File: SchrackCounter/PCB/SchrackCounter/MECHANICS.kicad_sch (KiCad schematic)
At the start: 24 parts, among them J3 Conn_01x02_Pin, J4 Conn_01x02_Pin, J5 MEM2067-02-180-00-A_REVB, M1 Fan_CPU_4pin, SW1 SW_Push, SW2 SW_Push, SW3 SW_Push, SW4 SW_Push

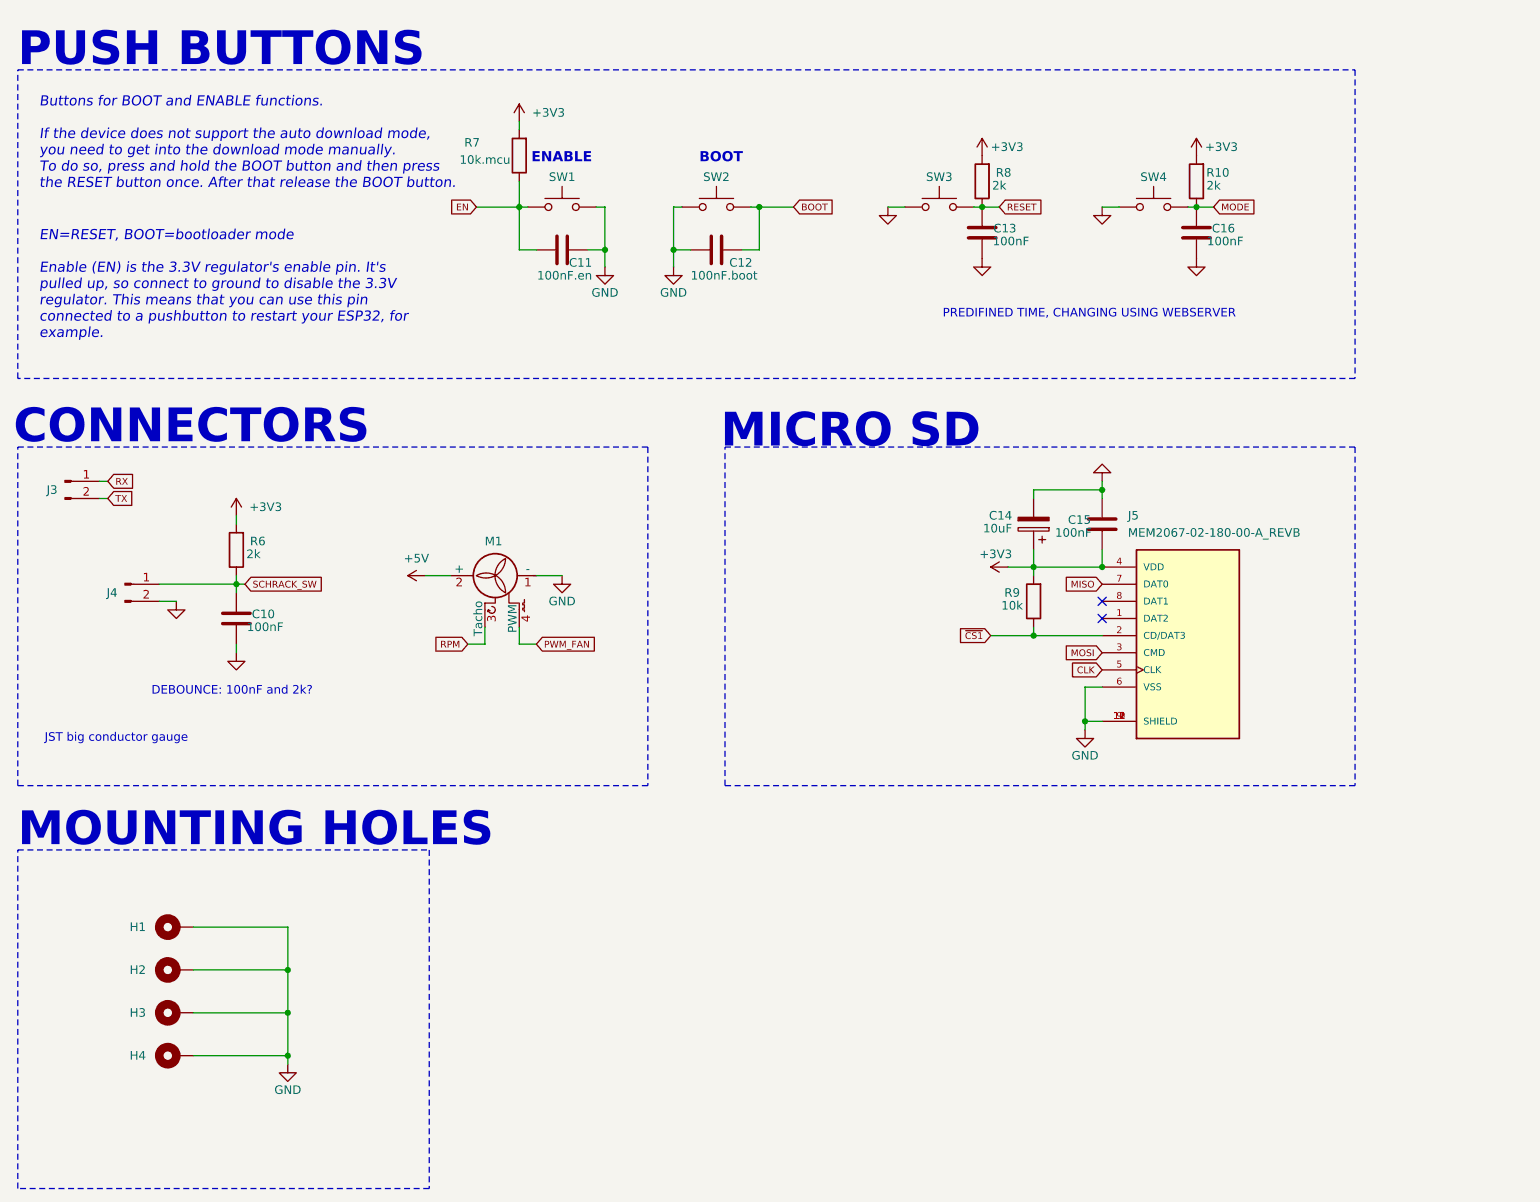
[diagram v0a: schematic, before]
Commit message: PCB layout update
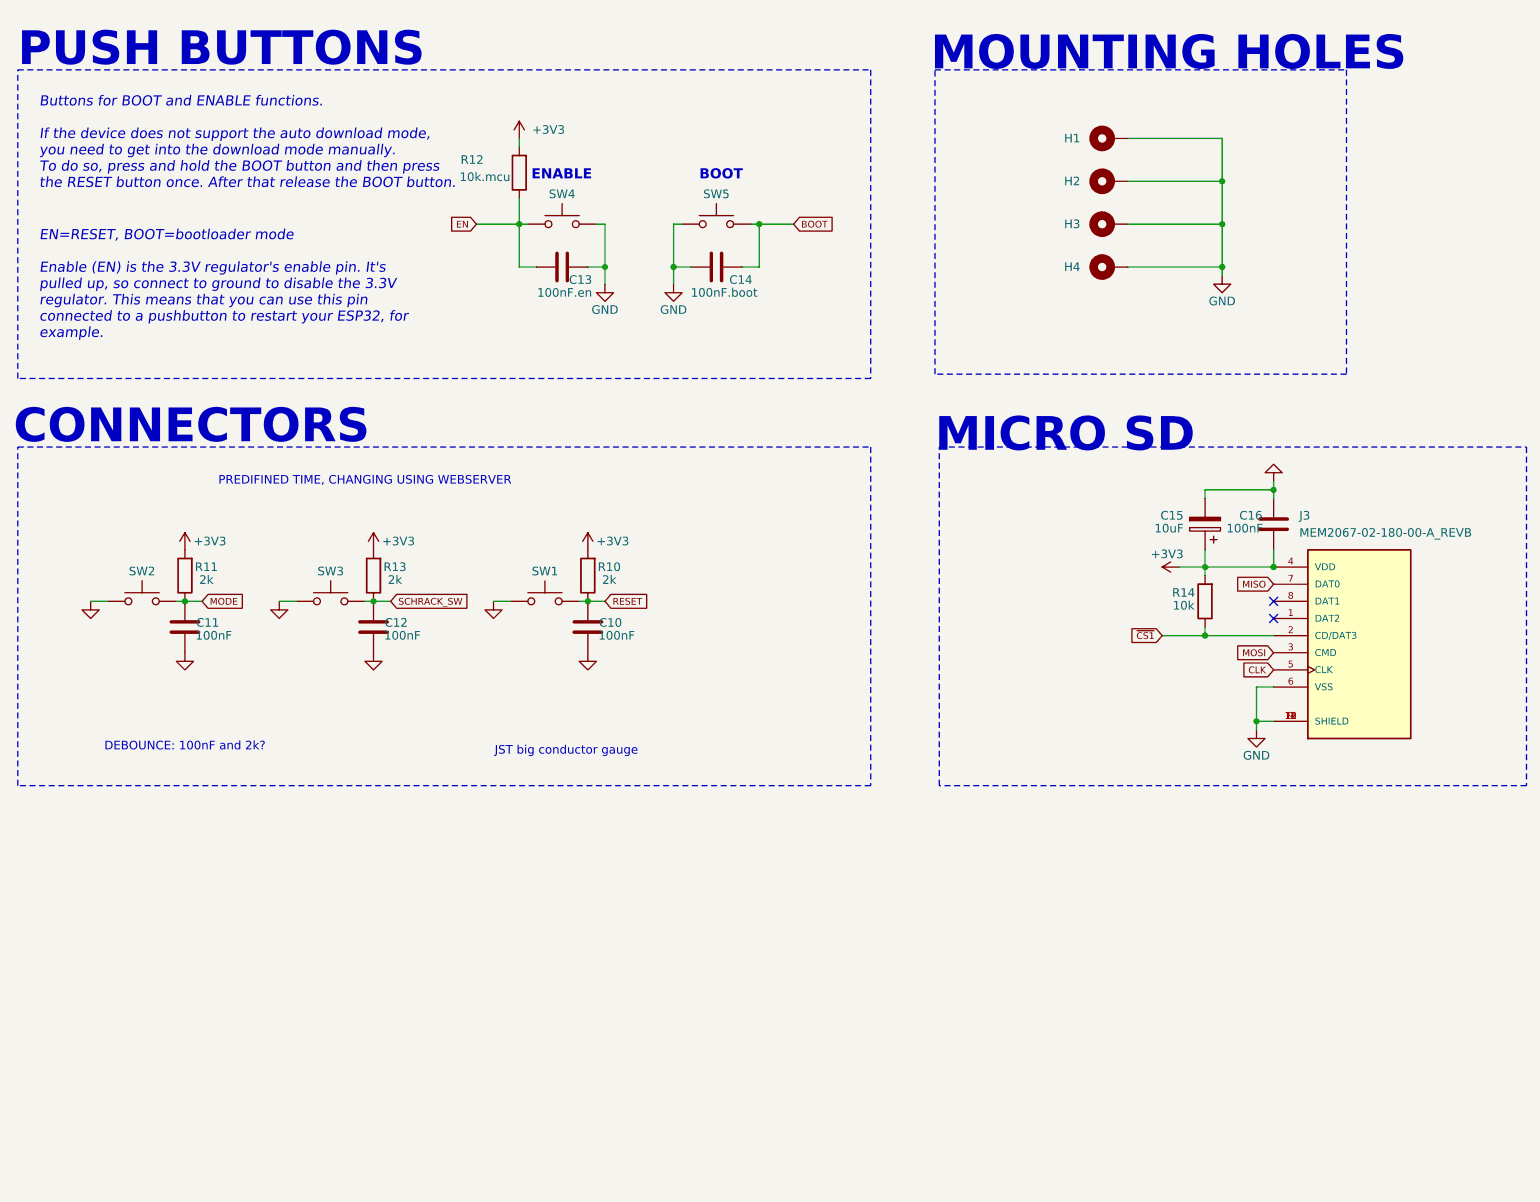
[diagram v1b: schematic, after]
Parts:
- removed J3: Conn_01x02_Pin, Connector_PinHeader_2.54mm:PinHeader_1x02_P2.54mm_Vertical, symbol Connector:Conn_01x02_Pin
- removed J4: Conn_01x02_Pin, Connector_JST:JST_XH_B2B-XH-A_1x02_P2.50mm_Vertical, symbol Connector:Conn_01x02_Pin
- removed M1: Fan_CPU_4pin, Connector:FanPinHeader_1x04_P2.54mm_Vertical, symbol Motor:Fan_CPU_4pin
- added SW3: SW_Push, Connector_JST:JST_XH_B2B-XH-A_1x02_P2.50mm_Vertical, symbol Switch:SW_Push
- renumbered C13 to C10, C16 to C11, C10 to C12, C11 to C13, C12 to C14, C14 to C15, C15 to C16, J5 to J3, R8 to R10, R10 to R11, R7 to R12, R6 to R13, R9 to R14, SW3 to SW1, SW4 to SW2, SW1 to SW4, SW2 to SW5
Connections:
- net GND: now also SW3.1
- net SCHRACK_SW: now also SW3.2
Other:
- moved on the sheet: C10, C11, C12, C13, C14, C15, C16, H1, H2, H3, H4, J3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
